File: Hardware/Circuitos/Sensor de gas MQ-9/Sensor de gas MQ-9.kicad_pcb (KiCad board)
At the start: 2 copper layers, 5 parts, among them J1 Conn_01x04, J2 Conn_01x02, J3 Conn_01x01

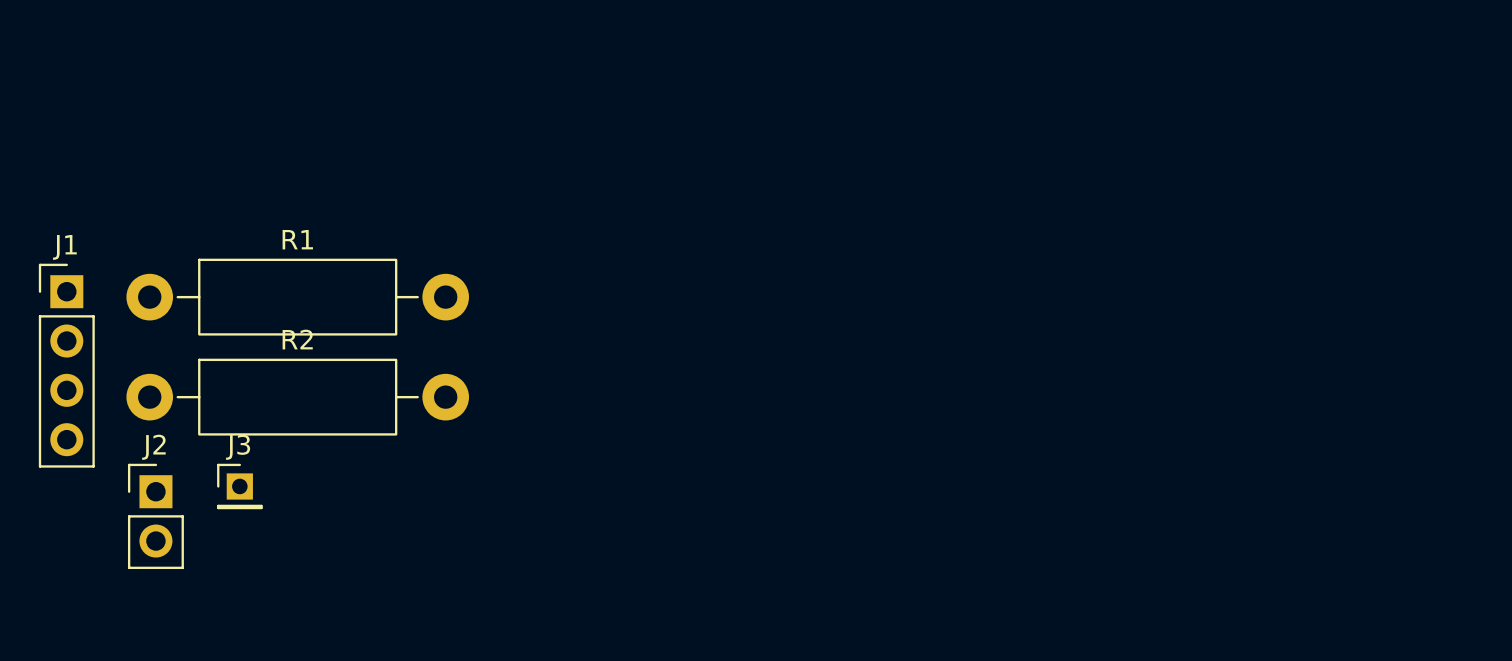
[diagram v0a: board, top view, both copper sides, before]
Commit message: Placa MQ9 - Colocación de componentes
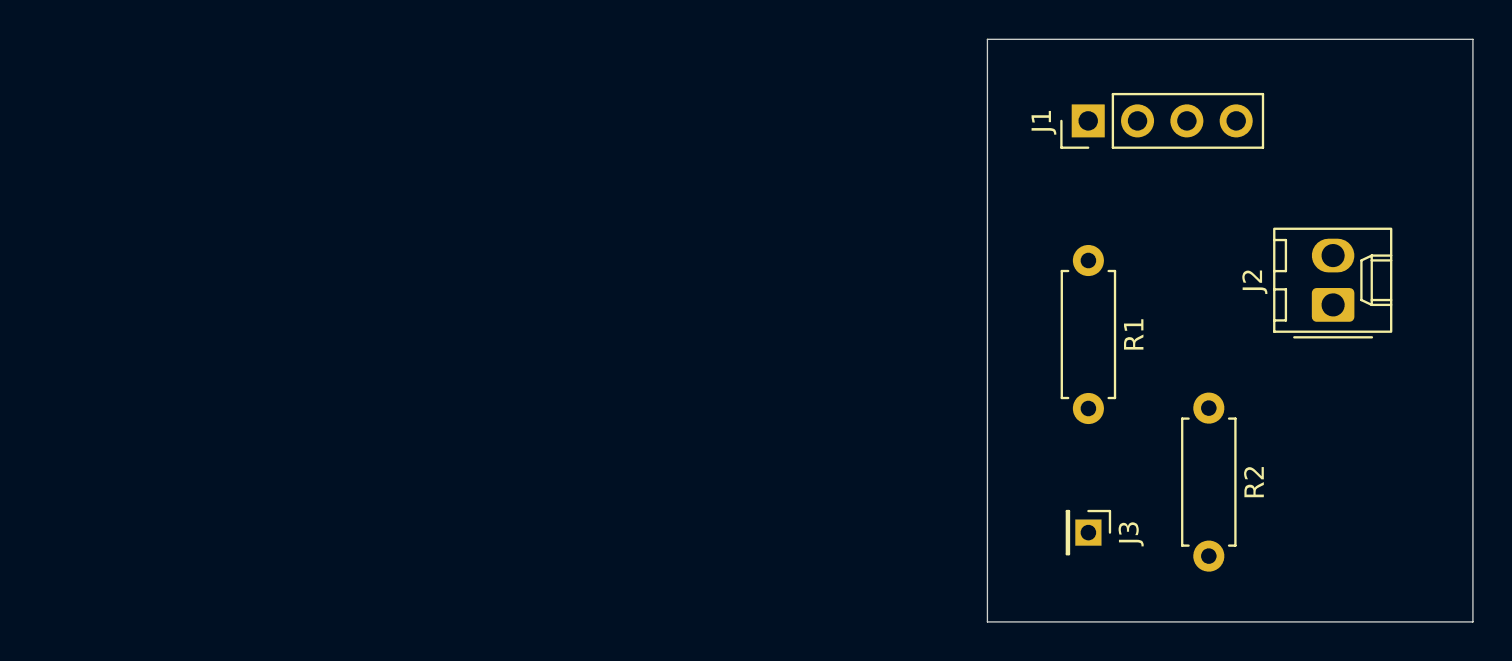
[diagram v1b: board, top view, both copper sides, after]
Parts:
- J2: footprint Connector_PinHeader_2.54mm:PinHeader_1x02_P2.54mm_Vertical -> Connector_Molex:Molex_KK-254_AE-6410-02A_1x02_P2.54mm_Vertical
- R1, R2: footprint Resistor_THT:R_Axial_DIN0411_L9.9mm_D3.6mm_P15.24mm_Horizontal -> Resistor_THT:R_Axial_DIN0207_L6.3mm_D2.5mm_P7.62mm_Horizontal
- moved J2 61.4 mm to (124.8, 62.1), turned to 90 degrees
- moved R2 54.5 mm to (118.4, 67.4), turned to -90 degrees
- moved J1 53.3 mm to (112.2, 52.6), turned to 90 degrees
- moved R1 48.4 mm to (112.2, 59.8), turned to -90 degrees
- moved J3 43.8 mm to (112.2, 73.8), turned to -90 degrees
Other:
- board outline added: 25 x 30 mm
